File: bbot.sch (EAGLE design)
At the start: 24 parts

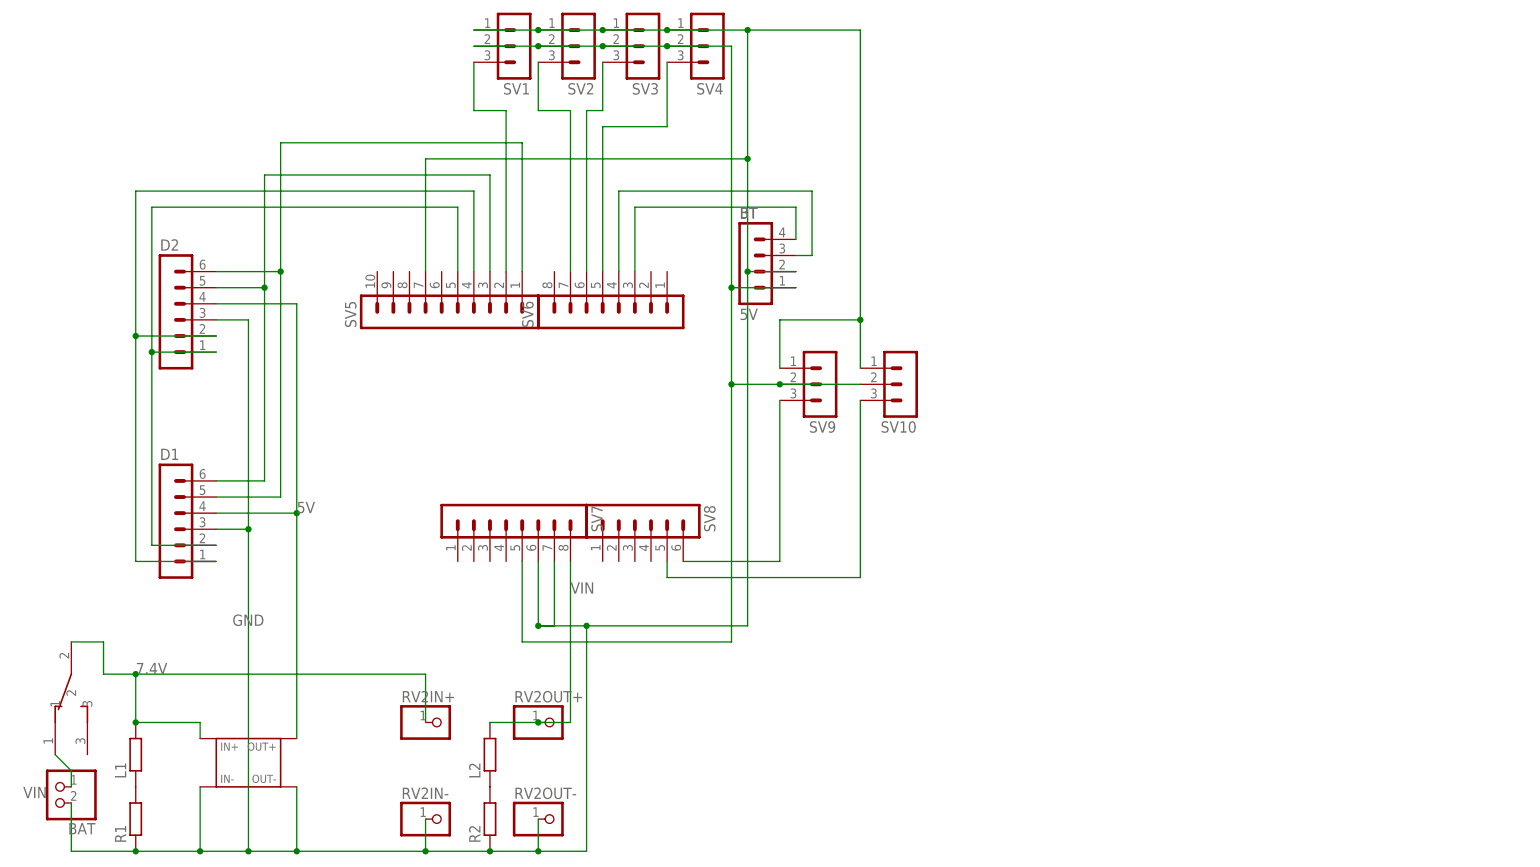
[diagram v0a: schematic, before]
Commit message: added some tags to brd
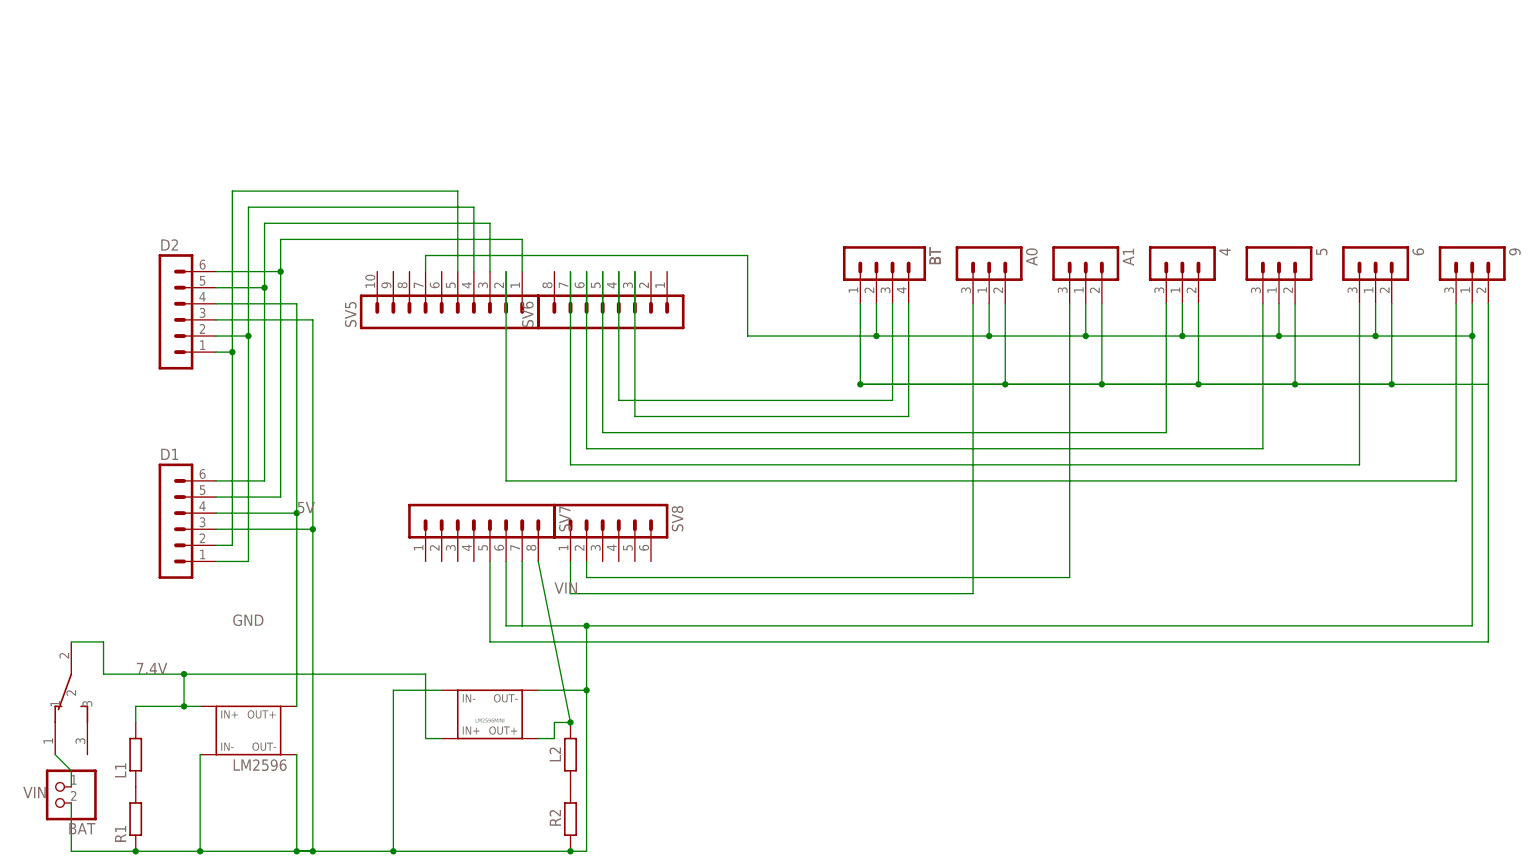
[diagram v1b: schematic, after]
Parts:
- removed RV2IN+, RV2IN-, RV2OUT+, RV2OUT-: (no value), adafruit:PINHD-1X1
- removed SV1, SV10, SV2, SV3, SV4, SV9: (no value), con-lstb:MA03-1
- removed U$1: BB-LM2596, my-library:BB-LM2596
- added 4, 5, 6, 9, A0, A1: BB-PIN3, my-library:BB-PIN3
- added LM2596: BB-LM2596, my-library:BB-LM2596
- added LM2596MINI: BB-LM2596MINI, my-library:BB-LM2596MINI
- BT: value 5V -> (none)
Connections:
- net 5V: now also LM2596.OUT+; no longer U$1.OUT+
- net 5V-A: now also 4.5V, 5.5V, 6.5V, 9.5V, A0.5V, A1.5V; no longer SV1.2, SV10.2, SV2.2, SV3.2, SV4.2, SV9.2
- net 7.4V: now also LM2596.IN+, LM2596MINI.IN+; no longer RV2IN+.1, U$1.IN+
- net GND: now also 4.GND, 5.GND, 6.GND, 9.GND, A0.GND, A1.GND, LM2596.IN-, LM2596.OUT-, LM2596MINI.IN-, LM2596MINI.OUT-; no longer RV2IN-.1, RV2OUT-.1, SV1.1, SV10.1, SV2.1, SV3.1, SV4.1, SV9.1, U$1.IN-, U$1.OUT-
- net N$14: now also 6.S; no longer SV2.3
- net N$15: now also 5.S; no longer SV3.3
- net N$16: now also 4.S; no longer SV4.3
- net N$17: now also A1.S, SV8.2; no longer SV8.6, SV9.3
- net N$18: now also A0.S, SV8.1; no longer SV10.3, SV8.5
- net N$5: now also 9.S; no longer SV1.3
- net VIN: now also LM2596MINI.OUT+; no longer RV2OUT+.1
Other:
- moved on the sheet: BT, L2, R2, SV7, SV8
